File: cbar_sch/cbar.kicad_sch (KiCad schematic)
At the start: 24 parts, among them J1 USB_C_Receptacle_PowerOnly_12V, SW1_PWR SW_SPST, SW2_TILT_TRIGGER SW_tilt, SW3_BATT_IND SW_Push, SW3_TILT_RESET SW_tilt, SW4_METAL SW_Push, SW5_BODY SW_Push

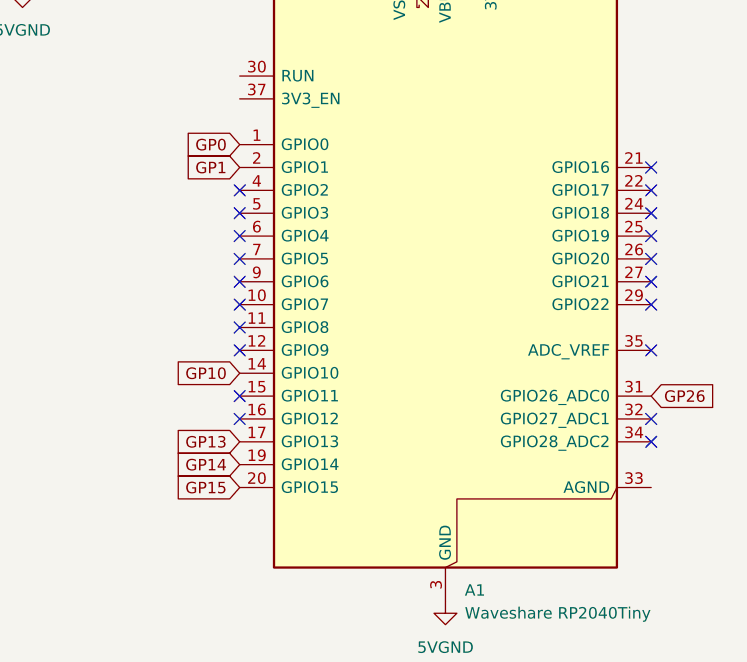
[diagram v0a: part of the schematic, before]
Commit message: Modeling
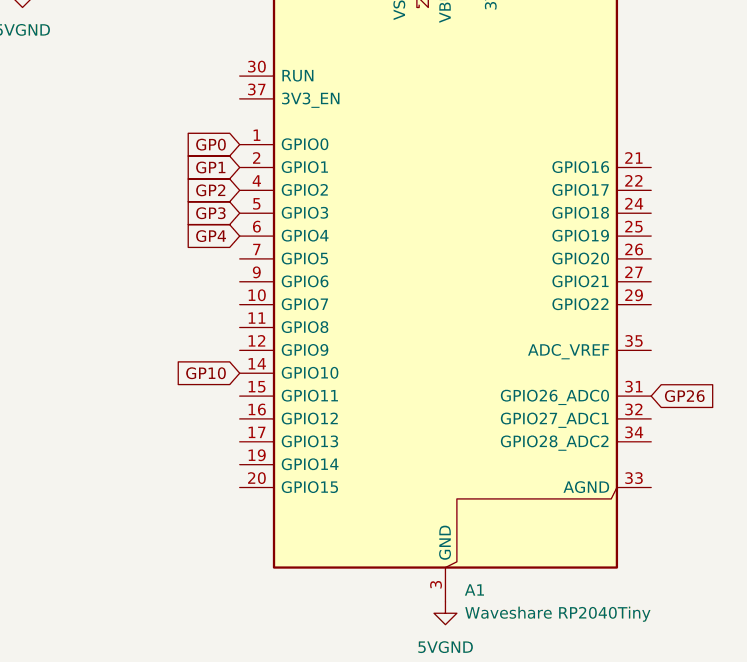
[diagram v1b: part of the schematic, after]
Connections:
- net GP13: no longer A1.17 (GPIO13)
- net GP14: no longer A1.19 (GPIO14)
- net GP15: no longer A1.20 (GPIO15)
- net GP2: now reaches A1.4 (GPIO2)
- net GP3: now reaches A1.5 (GPIO3)
- net GP4: now reaches A1.6 (GPIO4)
- no-connect marks 20 -> 0
